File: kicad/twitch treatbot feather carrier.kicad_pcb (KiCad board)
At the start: 2 copper layers, 33 parts, among them J1 128x64 OLED, J2 Quiic MP3 Trigger [CHECK FOOT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, J3 M2, J4 M1, J5 +12V_IN, J6 NEO_Signal, J7 +5V_IN, Q1 BSS138, SW1 ESP RESET, SW2 Wiggle, U1 TMC2208_BREAKOUT

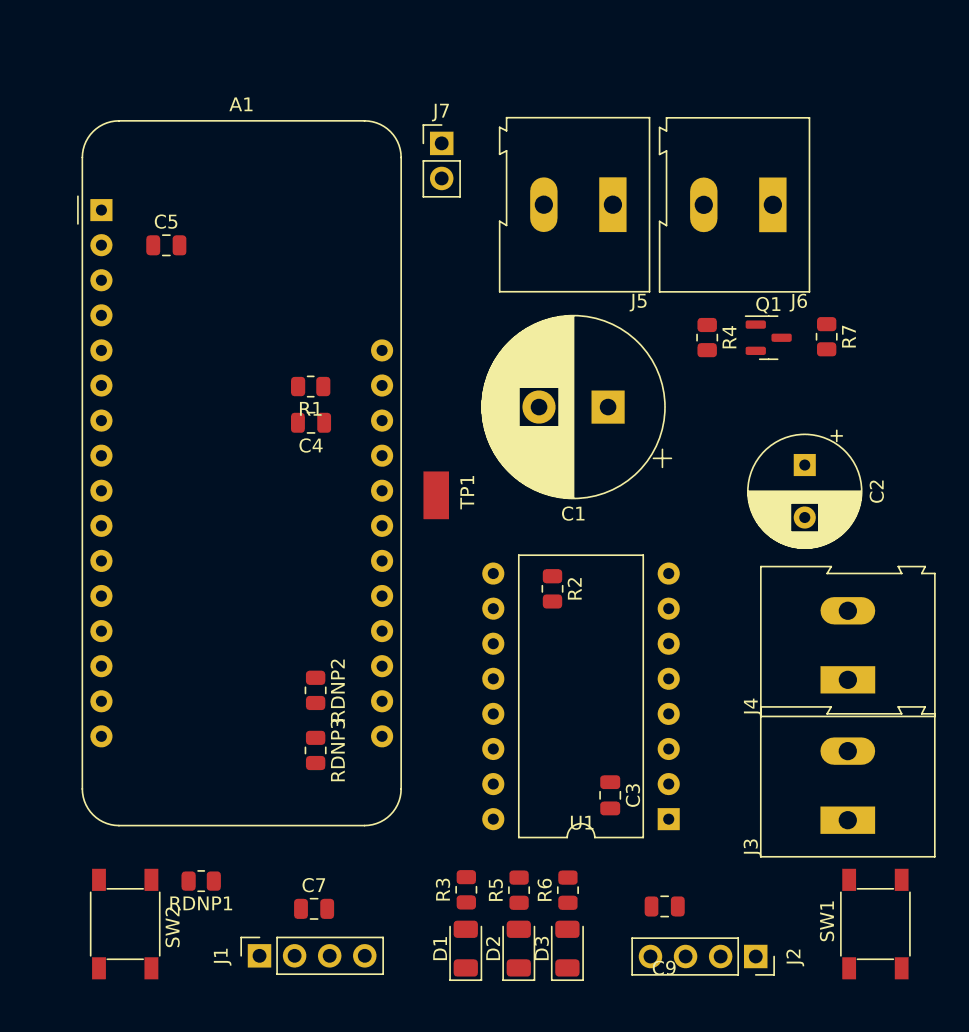
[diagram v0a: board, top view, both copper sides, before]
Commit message: 2nd floorplan
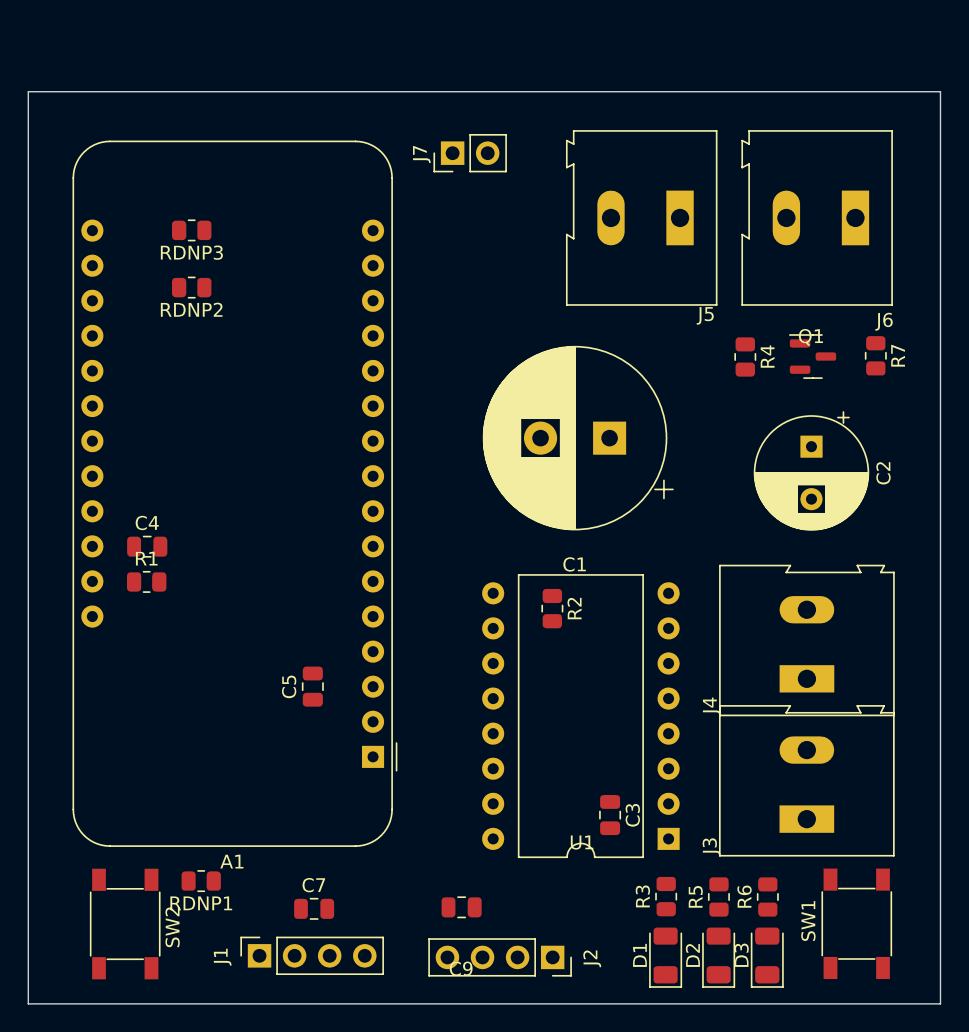
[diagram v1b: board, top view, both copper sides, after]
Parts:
- removed TP1: TestPoint_Harwin, My Libraries:Harwin-S1751-46-Test-Point
- moved A1 44.2 mm to (74.5, 104.0), turned to 180 degrees
- moved RDNP3 38.7 mm to (61.4, 65.9), turned to 180 degrees
- moved C5 33.7 mm to (70.1, 99.0), turned to 90 degrees
- moved RDNP2 30.5 mm to (61.4, 70.1), turned to 180 degrees
- moved R1 18.5 mm to (58.1, 91.4), turned to 0 degrees
- moved C4 14.9 mm to (58.1, 88.8), turned to 0 degrees
- moved C9 14.7 mm to (80.9, 114.9)
- moved J2 14.7 mm to (87.5, 118.6)
- moved D1 14.5 mm to (95.7, 118.4)
- moved D2 14.5 mm to (99.5, 118.4)
- moved D3 14.5 mm to (103.0, 118.4)
- moved R3 14.5 mm to (95.7, 114.2)
- moved R5 14.5 mm to (99.5, 114.2)
- moved R6 14.5 mm to (103.1, 114.2)
- moved J6 6.05 mm to (109.4, 65.0)
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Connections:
- A1 pad 11: /NEO_3v -> /STEP_DIR
- A1 pad 12: unconnected-(A1-Pad12) -> /STEP_STEP
- A1 pad 13: unconnected-(A1-Pad13) -> /STEP_EN
- A1 pad 15: unconnected-(A1-Pad15) -> /NEO_3v
- A1 pad 19: /STEP_EN -> unconnected-(A1-Pad19)
- A1 pad 20: /STEP_DIR -> unconnected-(A1-Pad20)
- A1 pad 22: /STEP_STEP -> unconnected-(A1-Pad22)
- A1 pad 23: /Wiggle -> unconnected-(A1-Pad23)
- A1 pad 24: Net-(A1-Pad24) -> unconnected-(A1-Pad24)
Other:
- board outline added: 66 x 66 mm

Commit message: Layout done, fully routed, most of silk done, debating if to convert to 2 layer board
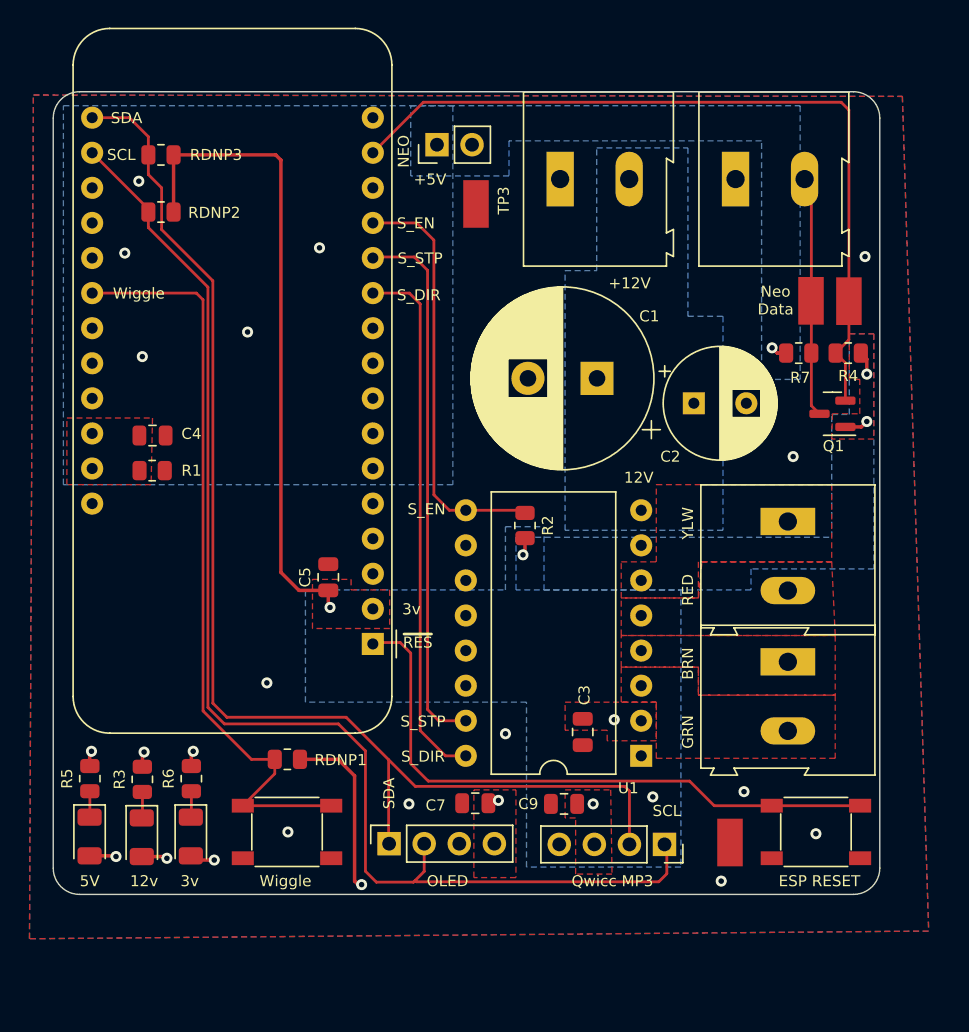
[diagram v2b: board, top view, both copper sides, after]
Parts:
- added TP1: TestPoint_Harwin, My Libraries:Harwin-S1751-46-Test-Point, F.Cu at (108.9, 71.0)
- added TP2: TestPoint_Harwin, My Libraries:Harwin-S1751-46-Test-Point, F.Cu at (106.2, 71.0)
- added TP3: TestPoint_Harwin, My Libraries:Harwin-S1751-46-Test-Point, F.Cu at (81.9, 64.0)
- added TP4: TestPoint_Harwin, My Libraries:Harwin-S1751-46-Test-Point, F.Cu at (100.3, 110.2)
- moved D2 46.4 mm to (54.0, 109.8), turned to -90 degrees
- moved R5 46.3 mm to (54.0, 105.6)
- moved D3 42.6 mm to (61.3, 109.8), turned to -90 degrees
- moved R6 42.6 mm to (61.3, 105.6)
- moved D1 38.9 mm to (57.7, 109.9), turned to -90 degrees
- moved R3 38.9 mm to (57.8, 105.7)
- moved C7 14.0 mm to (81.9, 107.4), turned to 180 degrees
- moved SW2 13.5 mm to (68.3, 109.5), turned to 0 degrees
- moved J1 12.4 mm to (75.7, 110.3)
- moved J2 11.5 mm to (95.6, 110.4)
- moved J4 11.5 mm to (104.5, 87.0), turned to -90 degrees
- moved J3 11.5 mm to (104.5, 97.2), turned to -90 degrees
- moved RDNP1 10.8 mm to (68.3, 104.2)
- moved C9 10.5 mm to (88.3, 107.4)
- moved J5 9.13 mm to (88.0, 62.2), turned to 0 degrees
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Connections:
- net Net-(A1-Pad1) renamed /~{RESET}
- A1 pad 22: unconnected-(A1-Pad22) -> /Wiggle
- J1 pad 4: /5V -> +5V
- J2 pad 3: /3v3 -> +3V3
- J3 pad 1: /M2B -> /M2A
- J3 pad 2: /M2A -> /M2B
- J4 pad 1: /M1A -> /M1B
- J4 pad 2: /M1B -> /M1A
- J5 pad 1: +12V -> GND
- J5 pad 2: GND -> +12V
- J6 pad 1: /NEO_5v -> GND
- J6 pad 2: GND -> /NEO_5v
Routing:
- net /SCL: track 0.00 -> 92.7 mm
- net /SDA: track 0.00 -> 90.3 mm
- net +3V3: track 0.00 -> 82.4 mm, vias 0 -> 7
- net +12V: track 0.00 -> 59.9 mm, vias 0 -> 1
- net /NEO_3v: track 0.00 -> 58.0 mm
- net /Wiggle: track 0.00 -> 55.4 mm
- net +5V: track 0.00 -> 46.3 mm, vias 0 -> 4
- net /~{RESET}: track 0.00 -> 44.9 mm
- net /STEP_STEP: track 0.00 -> 39.3 mm
- net /STEP_DIR: track 0.00 -> 38.7 mm
- net /STEP_EN: track 0.00 -> 30.5 mm
- net /NEO_5v: track 0.00 -> 17.4 mm
- net GND: track 0.00 -> 3.36 mm, vias 0 -> 18
- net Net-(D2-Pad1): track 0.00 -> 1.94 mm
- net Net-(D3-Pad1): track 0.00 -> 1.90 mm
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- added copper zone on B.Cu, net +12V
- added copper zone on B.Cu, net +3V3
- added copper zone on F.Cu, net +3V3
- added copper zone on B.Cu, net +5V
- added copper zone on F.Cu, net +5V
- added copper zone on In2.Cu, net +5V
- added copper zone on F.Cu, net /M1A
- added copper zone on F.Cu, net /M1B
- added copper zone on F.Cu, net /M2A
- added copper zone on F.Cu, net /M2B
- added copper zone on B.Cu, net GND
- added copper zone on F.Cu, net GND
- added copper zone on In1.Cu, net GND
- added copper zone on In2.Cu, net GND
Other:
- board size 66 x 66 mm -> 59.8 x 58.1 mm
- copper layers 2 -> 4
- board text added: "+12V"
- board text added: "+5V"
- board text added: "12V"
- board text added: "12v"
- board text added: "3v"
- board text added: "5V"
- board text added: "BRN"
- board text added: "ESP RESET"
- board text added: "GRN"
- board text added: "NEO"
- board text added: "Neo Data"
- board text added: "OLED"
- board text added: "Qwicc MP3"
- board text added: "RED"
- board text added: "SCL"
- board text added: "SDA"
- board text added: "S_DIR"
- board text added: "S_EN"
- board text added: "S_STP"
- board text added: "Wiggle"
- board text added: "YLW"
- board text added: "~{RES}"
